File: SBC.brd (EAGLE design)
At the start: 140.3 x 67.3 mm, 42 parts, among them IC1 MAX3232CPE, IC2 74LS04N, IC3 74LS00N, IC5 NE555P, J1 POWER_JACKPTH, J2 COMPUTER-PERIPHERAL-POWERRA, J3 22-27-2021-02

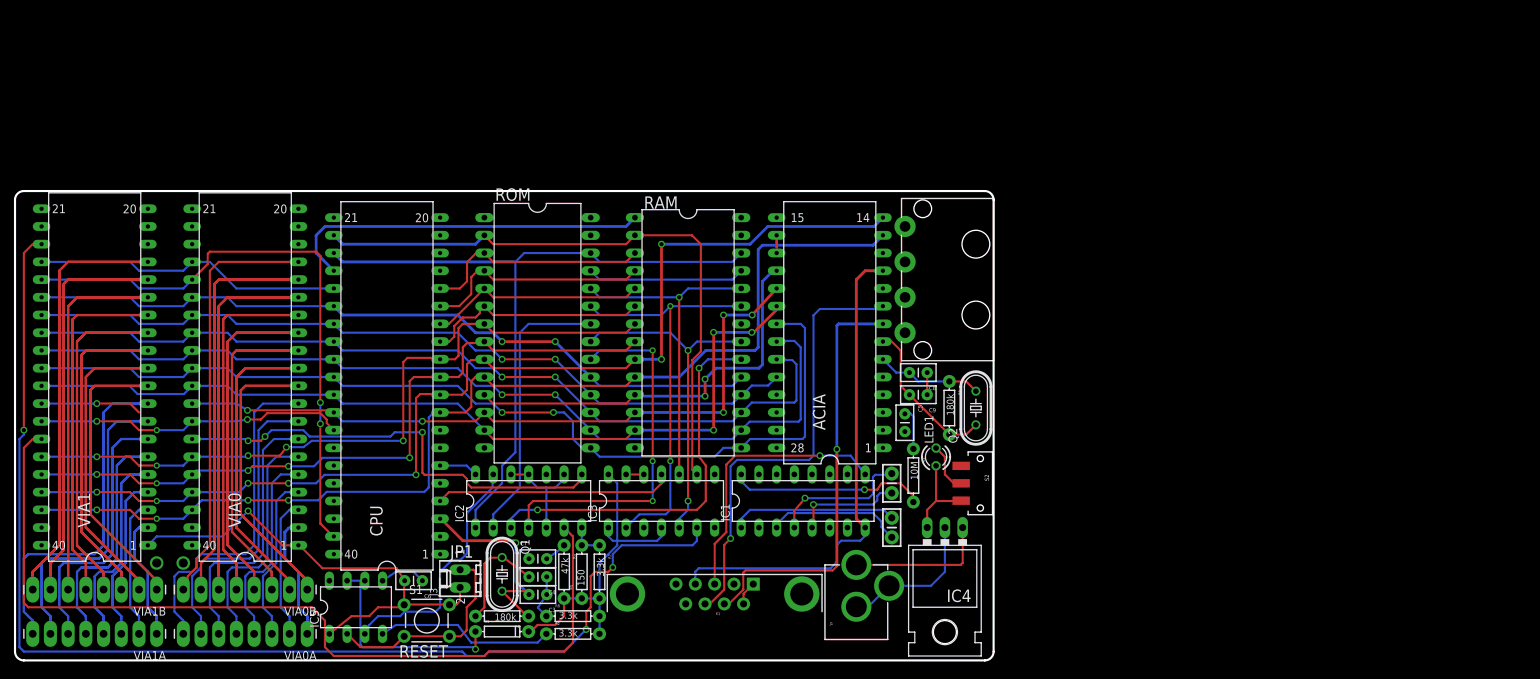
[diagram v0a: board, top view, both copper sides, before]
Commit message: Added gerber files
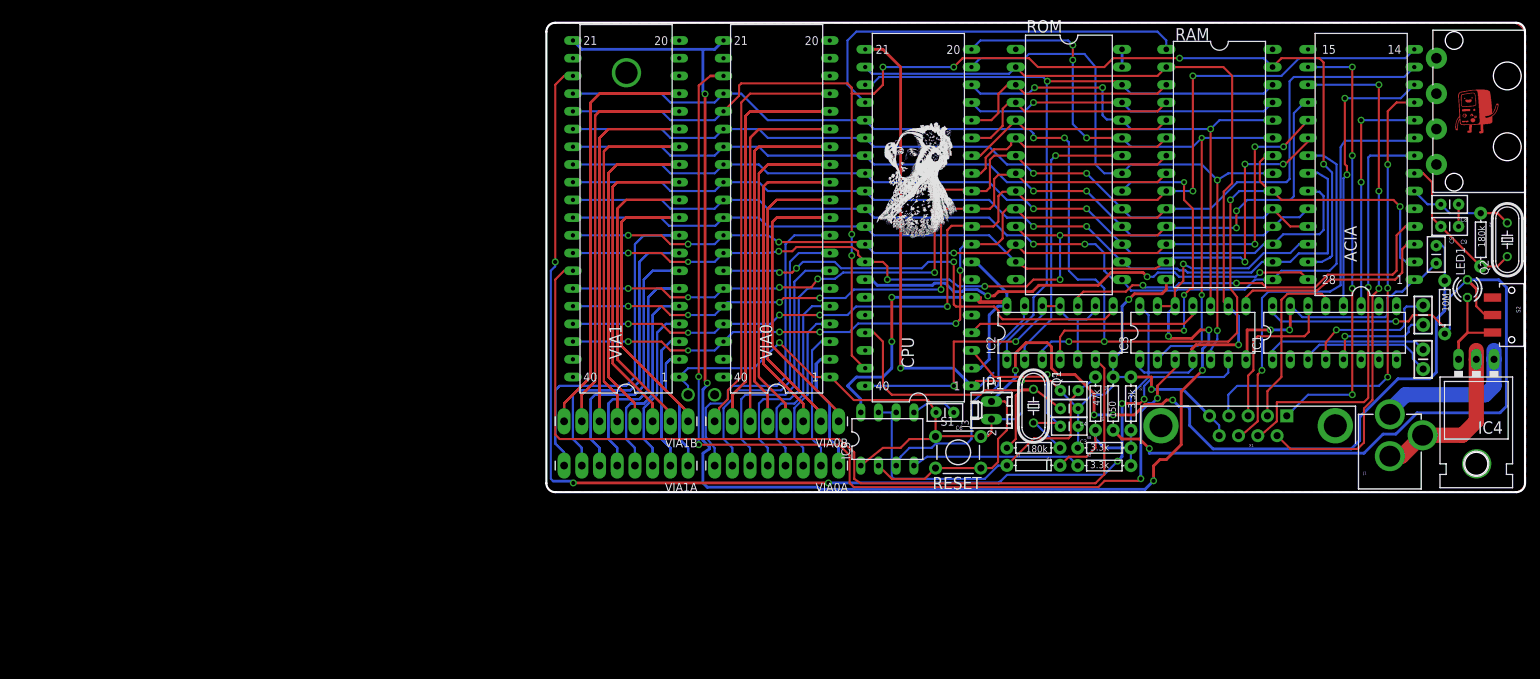
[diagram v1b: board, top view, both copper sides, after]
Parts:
- C7: value (none) -> 10uF
- RAM: value (none) -> 62256
- moved X1 80.2 mm to (187.0, 31.1)
- moved C1 79.9 mm to (212.1, 40.6)
- moved C2 79.9 mm to (212.1, 47.0)
- moved C3 79.9 mm to (162.6, 31.0)
- moved C4 79.9 mm to (162.6, 33.6)
- moved C5 79.9 mm to (214.0, 56.9)
- moved IC2 79.9 mm to (160.0, 44.5)
- moved IC4 79.9 mm to (219.7, 36.8)
- moved VIA0A 79.9 mm to (128.3, 25.4)
- moved VIA0B 79.9 mm to (128.3, 31.8)
- moved C6 79.9 mm to (144.8, 33.0)
- moved J3 79.9 mm to (150.2, 33.3)
- moved Q1 79.9 mm to (156.2, 33.9)
- moved R1 79.9 mm to (156.2, 27.9)
- moved R2 79.9 mm to (166.4, 25.4)
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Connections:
- removed net N$32: IC1.11
- removed net N$33: ACIA.5, IC1.14
- removed net RINGINDICATOR: X1.9
- removed net TRANSMITDATA: IC1.9, X1.3
- removed net VSS: RAM.14
- new net DATASETREADY: ACIA.17, X1.6
- new net N$1: LED1.K, R5.P$1
- new net N$3: IC1.14, X1.3
- new net N$5: ACIA.28, CPU.34
- new net N$7: ACIA.10, IC1.11
- new net N$8: ACIA.12, IC1.12
- net DATACARRIERDETECT: now also ACIA.16; no longer X1.6
- net DTEREADY: no longer IC1.8
- net GND: now also RAM.14, X1.9; no longer ACIA.16, ACIA.17
- net IRQ: now also ACIA.26, VIA0.21
- net N$17: now also VIA0.23
- net RECEIVEDATA: now also IC1.13
- net VCC: no longer LED1.K, R5.P$1
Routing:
- net IRQ: track 2.54 -> 216.9 mm, vias 0 -> 7
- net GND: track 107.6 -> 284.4 mm, vias 2 -> 8
- net N$17: track 0.00 -> 143.8 mm, vias 0 -> 4
- net PHI2: track 84.9 -> 190.4 mm, vias 2 -> 6
- net N$6: track 36.4 -> 138.9 mm, vias 0 -> 4
- net ADDRESS15: track 100.7 -> 199.9 mm, vias 2 -> 6
- net N$1: track 0.00 -> 84.0 mm, vias 0 -> 1
- net DATASETREADY: track 0.00 -> 76.0 mm, vias 0 -> 3
- net VCC: track 79.1 -> 153.5 mm, vias 2 -> 5
- net N$5: track 0.00 -> 67.7 mm, vias 0 -> 3
- net DATACARRIERDETECT: track 3.42 -> 64.0 mm, vias 0 -> 4
- net N$26: track 0.00 -> 57.5 mm, vias 0 -> 2
- net N$8: track 0.00 -> 40.9 mm, vias 0 -> 2
- net TRANSMITDATA: track 39.6 -> 0.00 mm, vias 1 -> 0
- net ADDRESS10: track 49.6 -> 87.0 mm
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- added copper zone on layer 16, net GND
- added copper zone on layer 1, net VCC
